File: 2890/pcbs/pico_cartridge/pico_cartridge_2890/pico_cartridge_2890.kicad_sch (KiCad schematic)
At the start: 55 parts, among them J1 Conn_01x12_Pin, J2 DIN41612_02x32_AB_acorn-syste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, J5 Conn_01x04_Female, SW1 A, SW2 A, SW7 A

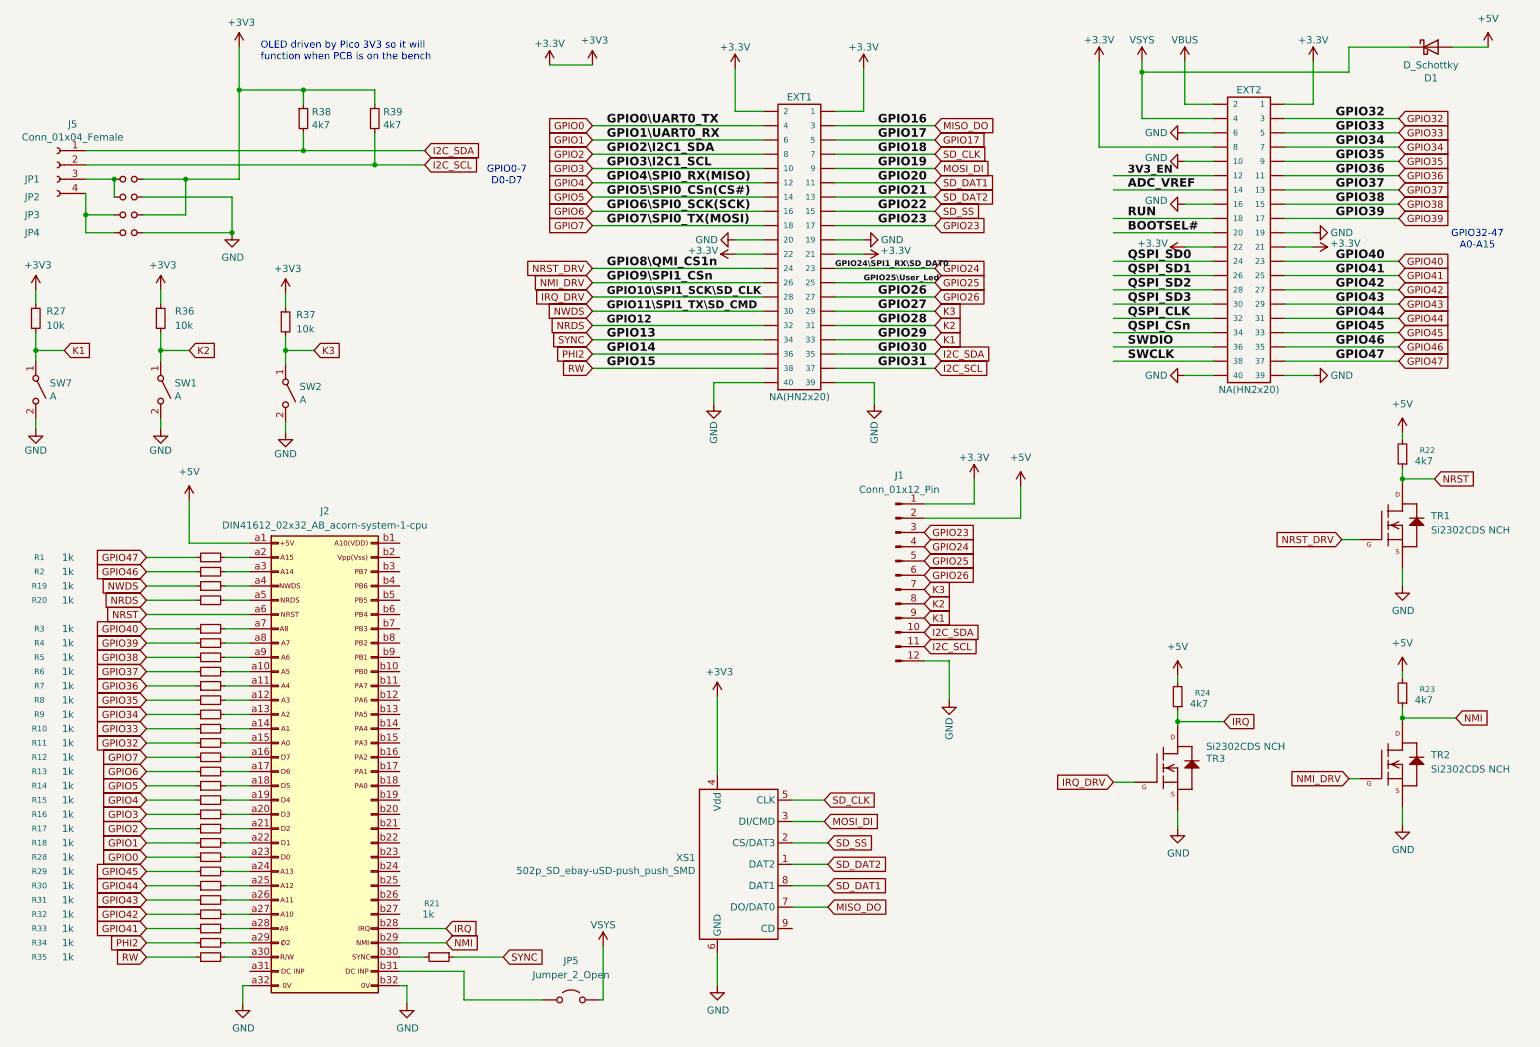
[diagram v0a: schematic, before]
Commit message: "Update"
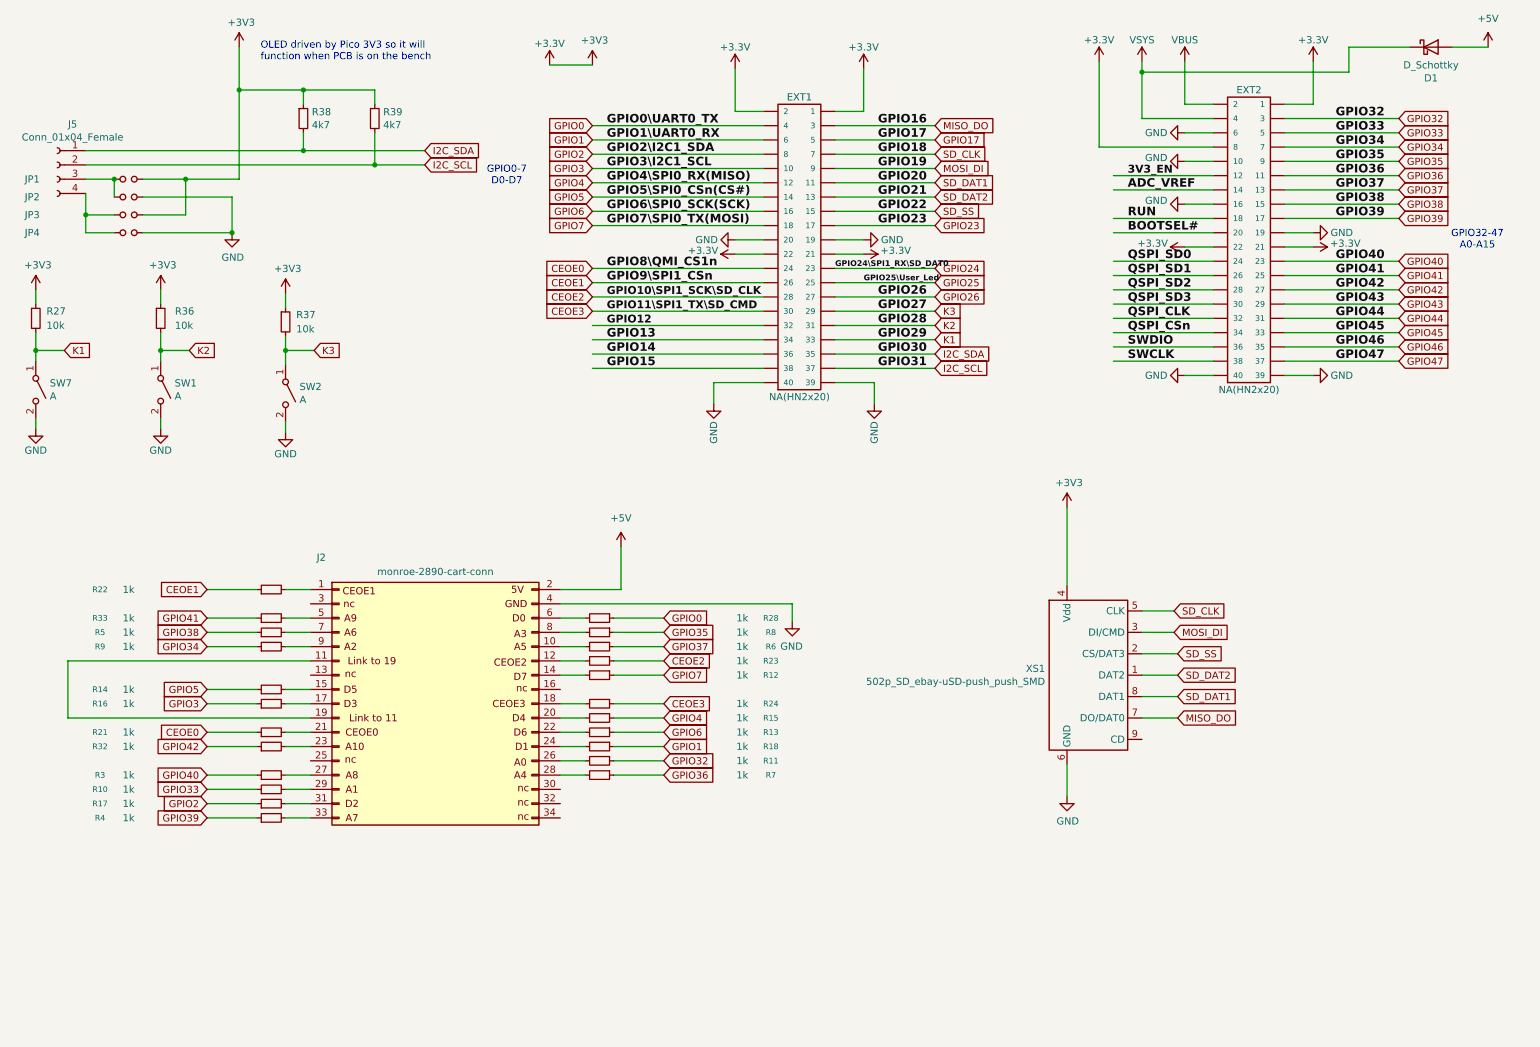
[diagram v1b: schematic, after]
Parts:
- removed J1: Conn_01x12_Pin, Connector_PinHeader_2.54mm:PinHeader_1x12_P2.54mm_Vertical, symbol Connector:Conn_01x12_Pin
- removed J2: DIN41612_02x32_AB_acorn-system-1-cpu, ajm-acorn:DIN41612_Q_2x32_Female_Horizontal_THT, symbol ajm-acorn-system-1:DIN41612_02x32_AB_acorn-system-1-cpu
- removed JP5: Jumper_2_Open, Connector_PinHeader_2.54mm:PinHeader_1x02_P2.54mm_Vertical, symbol Jumper:Jumper_2_Open
- removed R1, R19, R2, R20, R29, R30, R31, R34, R35: 1k, Resistor_SMD:R_0805_2012Metric_Pad1.20x1.40mm_HandSolder, symbol Device:R_Small
- removed TR1, TR2, TR3: Si2302CDS NCH, Package_TO_SOT_SMD:SOT-23, symbol ajm:Si2302CDS-n-channel
- added J2: monroe-2890-cart-conn, ajm-monroe:monroe-2890-cartridge-edge, symbol ajm-monroe:monroe-2890-cart-conn
- R22, R23, R24: value 4k7 -> 1k
- XS1: footprint ajm-acorn:Conn_uSDcard -> ajm-sdcard:Conn_uSDcard
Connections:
- net NMI is gone; now on net CEOE2: R23.1
- net NRST is gone; now on net CEOE1: R22.1
- net NWDS is gone; now on net CEOE3: EXT1.30
- net +5V: now also J2.2 (Pin_2); no longer R22.2, R23.2, R24.2
- net GND: now also J2.4 (Pin_4)
- net at R7.2: now also J2.28 (Pin_28)
- net at R8.2: now also J2.8 (Pin_8)
- net at R28.2: now also J2.6 (Pin_6)
- net at R12.2: now also J2.14 (Pin_14)
- net at R6.2: now also J2.10 (Pin_10)
- net at R15.2: now also J2.20 (Pin_20)
- net at R9.2: now also J2.9 (Pin_9)
- net at R10.2: now also J2.29 (Pin_29)
- net at R11.2: now also J2.26 (Pin_26)
- net at R13.2: now also J2.22 (Pin_22)
- net at R14.2: now also J2.15 (Pin_15)
- net at R16.2: now also J2.17 (Pin_17)
- net at R17.2: now also J2.31 (Pin_31)
- net at R18.2: now also J2.24 (Pin_24)
- net at R32.2: now also J2.23 (Pin_23)
- net at R33.2: now also J2.5 (Pin_5)
- net at R3.2: now also J2.27 (Pin_27)
- net at R4.2: now also J2.33 (Pin_33)
- net at R5.2: now also J2.7 (Pin_7)
- net at R21.2: now also J2.21 (Pin_21)
- net IRQ renamed CEOE3
- net IRQ_DRV renamed CEOE2
- net NMI_DRV renamed CEOE1
- net NRDS renamed GPIO12
- net NRST_DRV renamed CEOE0
- net CEOE0: now also R21.1
- net PHI2 renamed GPIO14
- net RW renamed GPIO15
- net SYNC renamed GPIO13
- net GPIO13: no longer R21.1
- new net: J2.12 (Pin_12), R23.2
- new net: J2.1 (Pin_1), R22.2
- new net: J2.11 (Pin_11), J2.19 (Pin_19)
- new net: J2.18 (Pin_18), R24.2
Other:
- moved on the sheet: R10, R11, R12, R13, R14, R15, R16, R17, R18, R28, R3, R32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
